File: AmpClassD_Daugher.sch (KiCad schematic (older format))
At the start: 73 parts, among them J1 POWER, J10 MONO, J11 LEFT, J12 INS, J13 OUTS, J14 PLIM_DEF, J2 POWER, J3 AUDIO_IN, J4 ST/MN, J5 GAIN_DEF, J6 SYNC_DEFAULT, J7 MN, J8 MN, J9 RIGHT, Q1 MMBT3904, Q2 MMBT3904, Q3 MMBT3904, Q4 MMBT3904, Q5 MMBT3904, U1 NE5532, U2 NE5532, U3 TPA3118D2

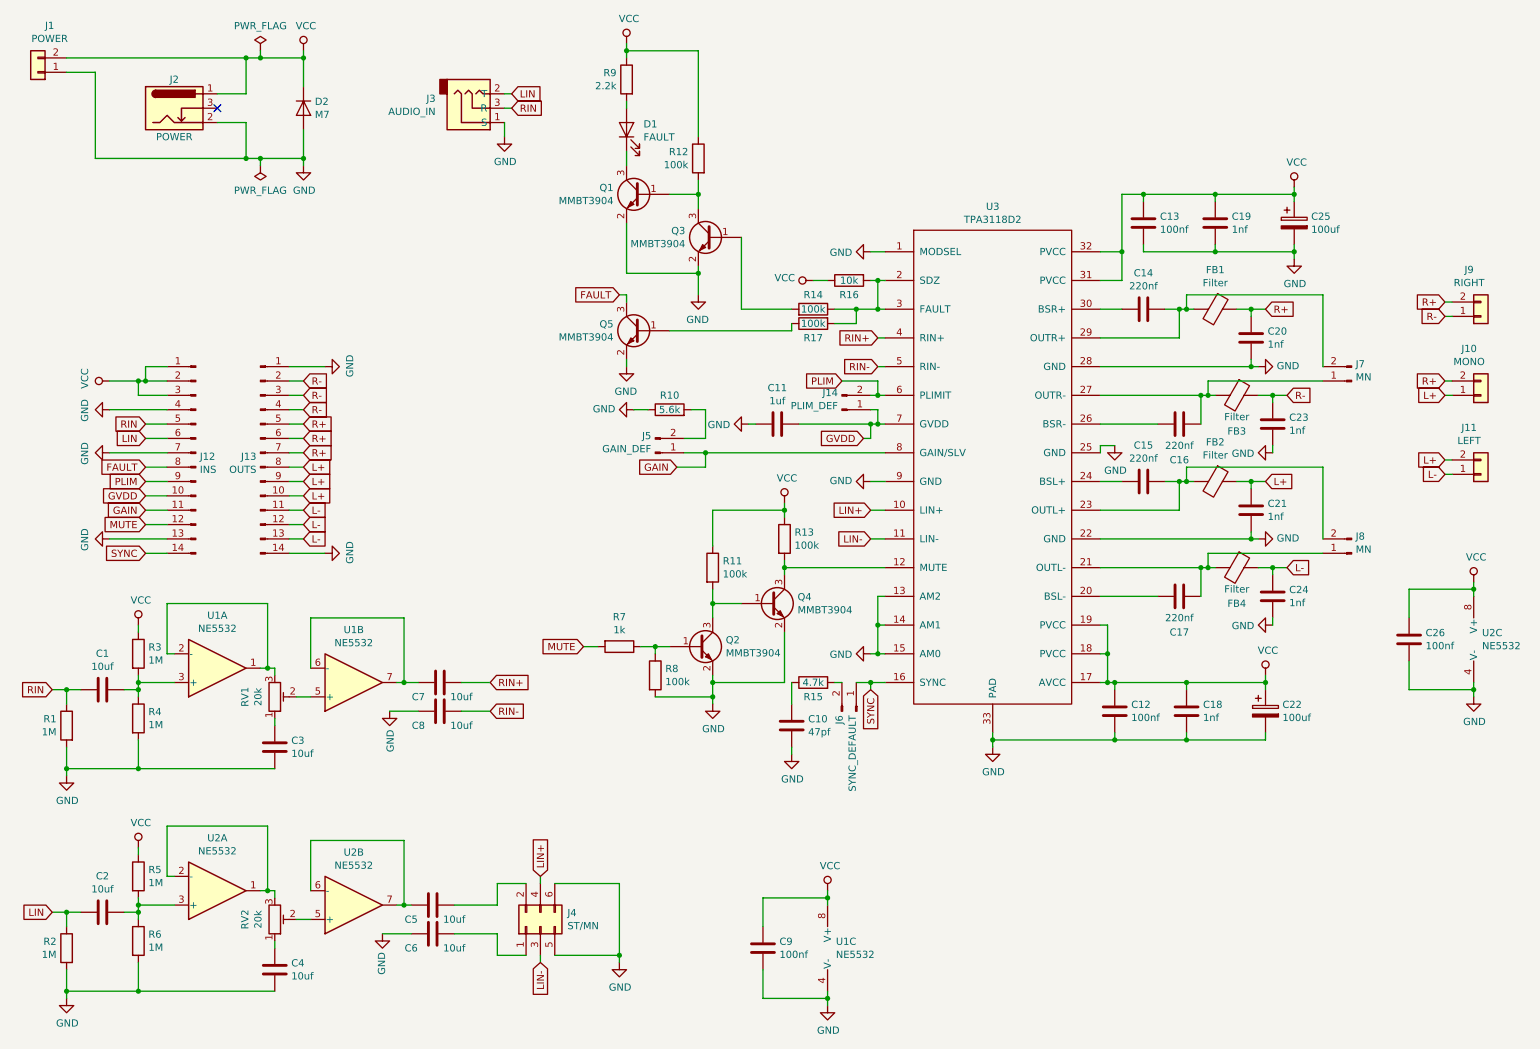
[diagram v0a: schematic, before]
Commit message: layout progress
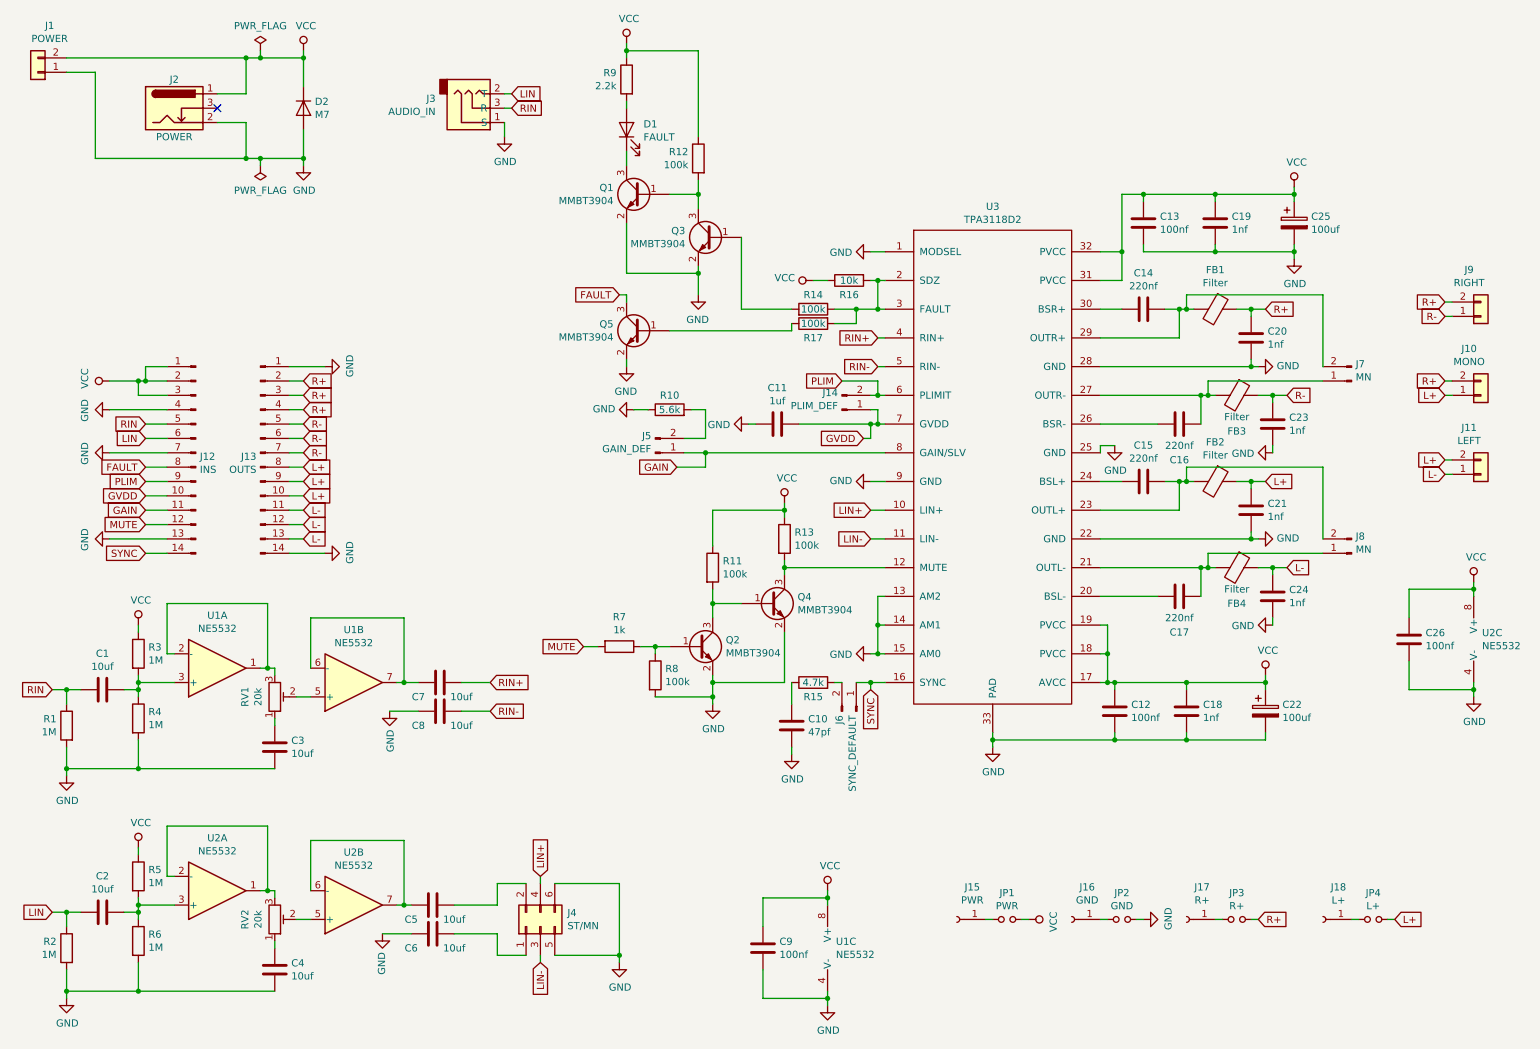
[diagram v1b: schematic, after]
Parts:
- added J15: PWR, HammerheadAudio:M3_Plated, symbol Connector:Conn_01x01_Female
- added J16: GND, HammerheadAudio:M3_Plated, symbol Connector:Conn_01x01_Female
- added J17: R+, HammerheadAudio:M3_Plated, symbol Connector:Conn_01x01_Female
- added J18: L+, HammerheadAudio:M3_Plated, symbol Connector:Conn_01x01_Female
- added JP1: PWR, Jumper:SolderJumper-2_P1.3mm_Open_Pad1.0x1.5mm, symbol Device:Jumper_NO_Small
- added JP2: GND, Jumper:SolderJumper-2_P1.3mm_Open_Pad1.0x1.5mm, symbol Device:Jumper_NO_Small
- added JP3: R+, Jumper:SolderJumper-2_P1.3mm_Open_Pad1.0x1.5mm, symbol Device:Jumper_NO_Small
- added JP4: L+, Jumper:SolderJumper-2_P1.3mm_Open_Pad1.0x1.5mm, symbol Device:Jumper_NO_Small
- J1, J10, J11, J9: footprint HammerheadAudio:Phoenix_Stacked_Marking2_Wider_NoRef -> HammerheadAudio:Phoenix_Stacked_Marking2_Wider_NoRef_Centered
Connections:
- net GND: now also JP2.2
- net L+: now also JP4.2
- net R+: now also J13.2 (Pin_2), J13.3 (Pin_3), J13.4 (Pin_4), JP3.2; no longer J13.5 (Pin_5), J13.6 (Pin_6), J13.7 (Pin_7)
- net R-: now also J13.5 (Pin_5), J13.6 (Pin_6), J13.7 (Pin_7); no longer J13.2 (Pin_2), J13.3 (Pin_3), J13.4 (Pin_4)
- net VCC: now also JP1.2
- new net: J15.1 (Pin_1), JP1.1
- new net: J16.1 (Pin_1), JP2.1
- new net: J17.1 (Pin_1), JP3.1
- new net: J18.1 (Pin_1), JP4.1
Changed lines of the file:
@@
 F 0 "J9" H 10668 2375 50  0000 C CNN
 F 1 "RIGHT" H 10668 2466 50  0000 C CNN
-F 2 "HammerheadAudio:Phoenix_Stacked_Marking2_Wider_NoRef" H 10750 2700 50  0001 C CNN
+F 2 "HammerheadAudio:Phoenix_Stacked_Marking2_Wider_NoRef_Centered" H 10750 2700 50  0001 C CNN
 F 3 "~" H 10750 2700 50  0001 C CNN
 	1    10750 2700
@@
 F 0 "J10" H 10668 2925 50  0000 C CNN
 F 1 "MONO" H 10668 3016 50  0000 C CNN
-F 2 "HammerheadAudio:Phoenix_Stacked_Marking2_Wider_NoRef" H 10750 3250 50  0001 C CNN
+F 2 "HammerheadAudio:Phoenix_Stacked_Marking2_Wider_NoRef_Centered" H 10750 3250 50  0001 C CNN
 F 3 "~" H 10750 3250 50  0001 C CNN
 	1    10750 3250
@@
 F 0 "J11" H 10668 3475 50  0000 C CNN
 F 1 "LEFT" H 10668 3566 50  0000 C CNN
-F 2 "HammerheadAudio:Phoenix_Stacked_Marking2_Wider_NoRef" H 10750 3800 50  0001 C CNN
+F 2 "HammerheadAudio:Phoenix_Stacked_Marking2_Wider_NoRef_Centered" H 10750 3800 50  0001 C CNN
 F 3 "~" H 10750 3800 50  0001 C CNN
 	1    10750 3800
@@
 F 0 "J1" H 618 675 50  0000 C CNN
 F 1 "POWER" H 618 766 50  0000 C CNN
-F 2 "HammerheadAudio:Phoenix_Stacked_Marking2_Wider_NoRef" H 700 1000 50  0001 C CNN
+F 2 "HammerheadAudio:Phoenix_Stacked_Marking2_Wider_NoRef_Centered" H 700 1000 50  0001 C CNN
 F 3 "~" H 700 1000 50  0001 C CNN
 	1    700  1000
@@
 	1    0    0    -1
 $EndComp
-Text GLabel 2550 3250 2    50   Input ~ 0
+Text GLabel 2550 3550 2    50   Input ~ 0
 R-
 Text GLabel 2550 3850 2    50   Input ~ 0
@@
 Text GLabel 2550 3750 2    50   Input ~ 0
 L+
-Text GLabel 2550 3650 2    50   Input ~ 0
+Text GLabel 2550 3350 2    50   Input ~ 0
 R+
 Wire Wire Line
@@
 Wire Wire Line
 	1450 3150 1400 3150
-Text GLabel 2550 3550 2    50   Input ~ 0
+Text GLabel 2550 3250 2    50   Input ~ 0
 R+
 Wire Wire Line
@@
 Wire Wire Line
 	2450 3550 2550 3550
-Text GLabel 2550 3350 2    50   Input ~ 0
+Text GLabel 2550 3650 2    50   Input ~ 0
 R-
 Wire Wire Line
@@
 Wire Wire Line
 	1450 4150 1600 4150
+Text GLabel 2550 3450 2    50   Input ~ 0
+R-
+Wire Wire Line
+	2450 3150 2550 3150
 Text GLabel 2550 3150 2    50   Input ~ 0
-R-
-Wire Wire Line
-	2450 3150 2550 3150
-Text GLabel 2550 3450 2    50   Input ~ 0
 R+
 Wire Wire Line
@@
 Wire Wire Line
 	2450 4350 2700 4350
+$Comp
+L Connector:Conn_01x01_Female J15
+U 1 1 6354D0B7
+P 7100 6900
+F 0 "J15" H 6992 6675 50  0000 C CNN
+F 1 "PWR" H 6992 6766 50  0000 C CNN
+F 2 "HammerheadAudio:M3_Plated" H 7100 6900 50  0001 C CNN
+F 3 "~" H 7100 6900 50  0001 C CNN
+	1    7100 6900
+	-1   0    0    1
+$EndComp
+$Comp
+L Connector:Conn_01x01_Female J16
+U 1 1 635549EB
+P 7900 6900
+F 0 "J16" H 7792 6675 50  0000 C CNN
+F 1 "GND" H 7792 6766 50  0000 C CNN
+F 2 "HammerheadAudio:M3_Plated" H 7900 6900 50  0001 C CNN
+F 3 "~" H 7900 6900 50  0001 C CNN
+	1    7900 6900
+	-1   0    0    1
+$EndComp
+$Comp
+L Device:Jumper_NO_Small JP1
+U 1 1 635554C5
+P 7450 6900
+F 0 "JP1" H 7450 7085 50  0000 C CNN
+F 1 "PWR" H 7450 6994 50  0000 C CNN
+F 2 "Jumper:SolderJumper-2_P1.3mm_Open_Pad1.0x1.5mm" H 7450 6900 50  0001 C CNN
+F 3 "~" H 7450 6900 50  0001 C CNN
+	1    7450 6900
+	1    0    0    -1
+$EndComp
+Wire Wire Line
+	7300 6900 7350 6900
+$Comp
+L power:VCC #PWR035
+U 1 1 63577A57
+P 7600 6900
+F 0 "#PWR035" H 7600 6750 50  0001 C CNN
+F 1 "VCC" H 7617 7073 50  0000 C CNN
+F 2 "" H 7600 6900 50  0001 C CNN
+F 3 "" H 7600 6900 50  0001 C CNN
+	1    7600 6900
+	0    1    1    0
+$EndComp
+Wire Wire Line
+	7550 6900 7600 6900
+$Comp
+L Device:Jumper_NO_Small JP2
+U 1 1 63599BCE
+P 8250 6900
+F 0 "JP2" H 8250 7085 50  0000 C CNN
+F 1 "GND" H 8250 6994 50  0000 C CNN
+F 2 "Jumper:SolderJumper-2_P1.3mm_Open_Pad1.0x1.5mm" H 8250 6900 50  0001 C CNN
+F 3 "~" H 8250 6900 50  0001 C CNN
+	1    8250 6900
+	1    0    0    -1
+$EndComp
+Wire Wire Line
+	8100 6900 8150 6900
+Wire Wire Line
+	8350 6900 8400 6900
+$Comp
+L power:GND #PWR036
+U 1 1 635BBA28
+P 8400 6900
+F 0 "#PWR036" H 8400 6650 50  0001 C CNN
+F 1 "GND" H 8405 6727 50  0000 C CNN
+F 2 "" H 8400 6900 50  0001 C CNN
+F 3 "" H 8400 6900 50  0001 C CNN
+	1    8400 6900
+	0    -1   -1   0
+$EndComp
+$Comp
+L Connector:Conn_01x01_Female J17
+U 1 1 635BC077
+P 8700 6900
+F 0 "J17" H 8592 6675 50  0000 C CNN
+F 1 "R+" H 8592 6766 50  0000 C CNN
+F 2 "HammerheadAudio:M3_Plated" H 8700 6900 50  0001 C CNN
+F 3 "~" H 8700 6900 50  0001 C CNN
+	1    8700 6900
+	-1   0    0    1
+$EndComp
+$Comp
+L Connector:Conn_01x01_Female J18
+U 1 1 635BC081
+P 9650 6900
+F 0 "J18" H 9542 6675 50  0000 C CNN
+F 1 "L+" H 9542 6766 50  0000 C CNN
+F 2 "HammerheadAudio:M3_Plated" H 9650 6900 50  0001 C CNN
+F 3 "~" H 9650 6900 50  0001 C CNN
+	1    9650 6900
+	-1   0    0    1
+$EndComp
+$Comp
+L Device:Jumper_NO_Small JP3
+U 1 1 635BC08B
+P 9050 6900
+F 0 "JP3" H 9050 7085 50  0000 C CNN
+F 1 "R+" H 9050 6994 50  0000 C CNN
+F 2 "Jumper:SolderJumper-2_P1.3mm_Open_Pad1.0x1.5mm" H 9050 6900 50  0001 C CNN
+F 3 "~" H 9050 6900 50  0001 C CNN
+	1    9050 6900
+	1    0    0    -1
+$EndComp
+Wire Wire Line
+	8900 6900 8950 6900
+Wire Wire Line
+	9150 6900 9200 6900
+$Comp
+L Device:Jumper_NO_Small JP4
+U 1 1 635BC0A1
+P 10000 6900
+F 0 "JP4" H 10000 7085 50  0000 C CNN
+F 1 "L+" H 10000 6994 50  0000 C CNN
+F 2 "Jumper:SolderJumper-2_P1.3mm_Open_Pad1.0x1.5mm" H 10000 6900 50  0001 C CNN
+F 3 "~" H 10000 6900 50  0001 C CNN
+	1    10000 6900
+	1    0    0    -1
+$EndComp
+Wire Wire Line
+	9850 6900 9900 6900
+Wire Wire Line
+	10100 6900 10150 6900
+Text GLabel 10150 6900 2    50   Input ~ 0
+L+
+Text GLabel 9200 6900 2    50   Input ~ 0
+R+
 $EndSCHEMATC
